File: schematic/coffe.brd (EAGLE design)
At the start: 87.3 x 48.2 mm, 18 parts, among them Q1 BC546B

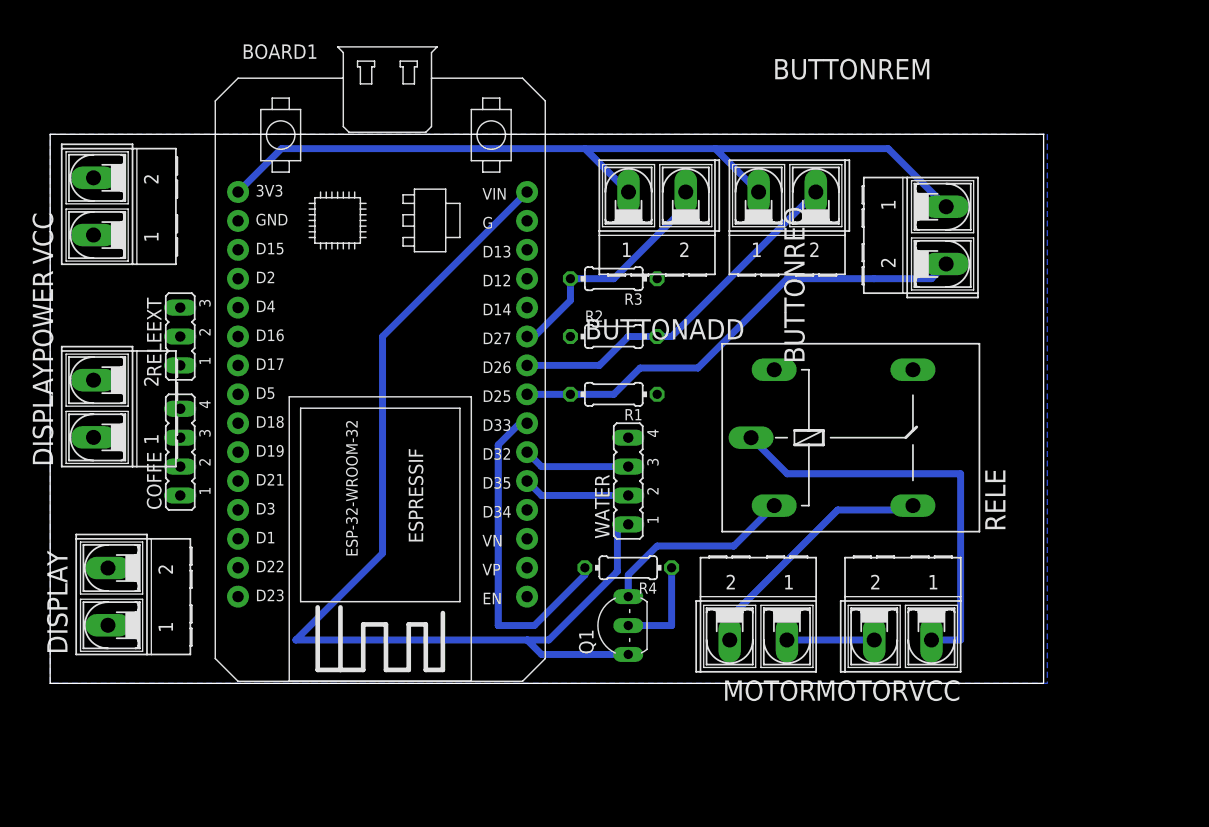
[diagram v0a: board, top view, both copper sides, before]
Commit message: Routing complete
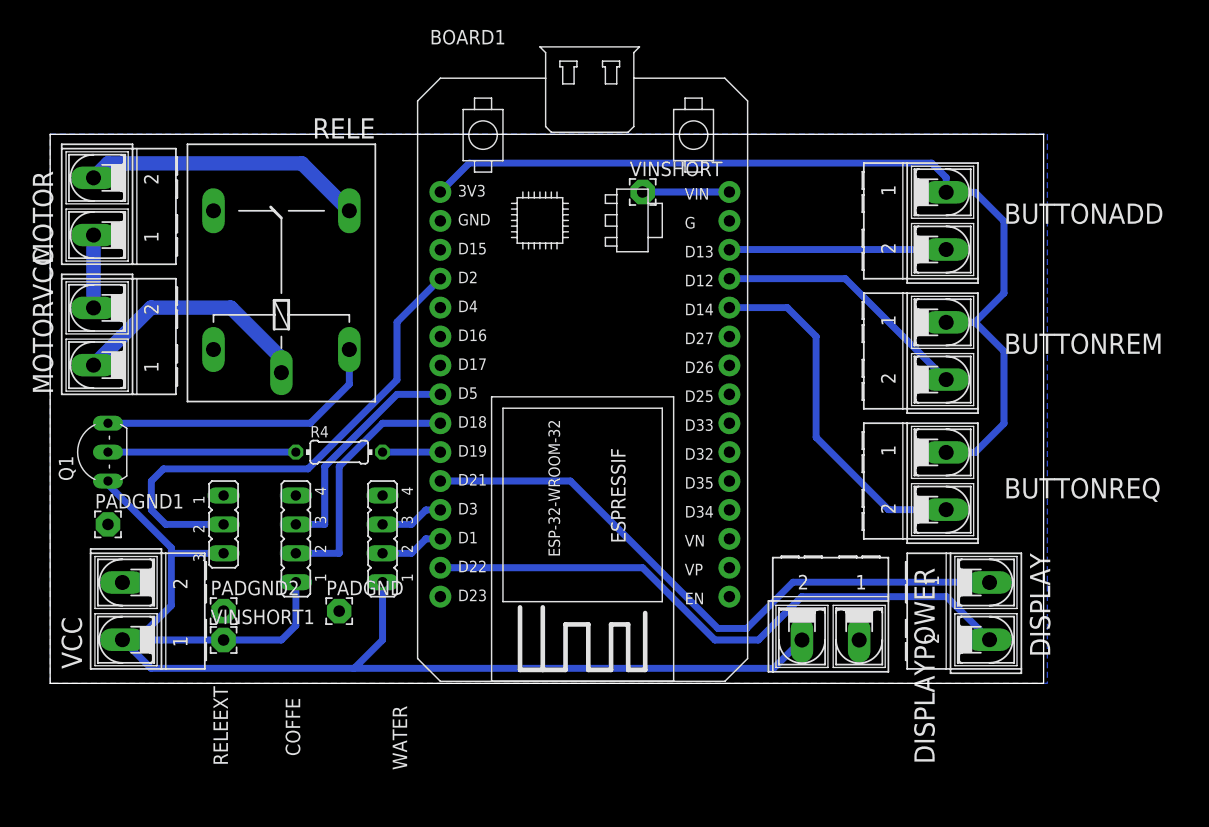
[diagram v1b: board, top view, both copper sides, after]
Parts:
- removed R1, R2, R3: 10K, rcl:0204/7
- added PADGND, PADGND1, PADGND2, VINSHORT, VINSHORT1: (no value), wirepad:2,15/1,0
- moved DISPLAY 77.5 mm to (82.5, 6.35), turned to 270 degrees
- moved MOTORVCC 76.0 mm to (3.81, 30.5), turned to 90 degrees
- moved MOTOR 69.7 mm to (3.81, 41.9), turned to 90 degrees
- moved DISPLAYPOWER 67.9 mm to (68.6, 3.81), turned to 180 degrees
- moved RELE 53.0 mm to (20.3, 36.8), turned to 90 degrees
- moved Q1 48.2 mm to (3.81, 20.3)
- moved VCC 35.7 mm to (6.35, 6.35)
- moved R4 27.4 mm to (25.4, 20.3), turned to 0 degrees
- moved BUTTONADD 25.5 mm to (78.7, 40.6), turned to 270 degrees
- moved WATER 22.2 mm to (29.2, 12.7)
- moved BUTTONREQ 21.6 mm to (78.7, 17.8)
- moved BUTTONREM 19.8 mm to (78.7, 29.2), turned to 270 degrees
- moved BOARD1 17.8 mm to (34.3, 43.2)
- moved RELEEXT 16.9 mm to (15.2, 14.0), turned to 270 degrees
- moved COFFE 12.7 mm to (21.6, 12.7)
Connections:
- removed net N$7 (its old number): BOARD1.D33, R4.2
- new net N$5: BOARD1.D14, BUTTONREQ.2
- net GND: now also BOARD1.GND@1, PADGND.1, PADGND1.1, PADGND2.1; no longer R1.1, R2.1, R3.1
- net N$1: now also BOARD1.D3; no longer BOARD1.D32
- net N$16: now also BOARD1.D13; no longer BOARD1.D27, R3.2
- net N$18: now also BOARD1.D12; no longer BOARD1.D26, R2.2
- net N$2: now also BOARD1.D1; no longer BOARD1.D35
- net N$6: now also BOARD1.D19, R4.2; no longer BOARD1.D25, BUTTONREQ.2, R1.2
- net VCC: now also VINSHORT.1, VINSHORT1.1
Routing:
- net N$17: track 0.00 -> 55.3 mm
- net N$8: track 0.00 -> 54.0 mm
- net N$14: track 0.00 -> 45.2 mm
- net N$6: track 41.6 -> 5.08 mm
- net N$5: track 0.00 -> 31.6 mm
- net N$7 (its old number): track 29.3 -> 0.00 mm
- net VCC: track 92.9 -> 121.0 mm
- net N$4: track 0.00 -> 21.9 mm
- net N$3: track 0.00 -> 20.4 mm
- net N$13: track 36.9 -> 21.7 mm
- net N$18: track 31.7 -> 22.7 mm
- net N$10: track 17.3 -> 25.7 mm
- net N$7: track 76.7 -> 84.5 mm
- net N$9: track 8.89 -> 16.5 mm
- net N$2: track 9.42 -> 5.61 mm
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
